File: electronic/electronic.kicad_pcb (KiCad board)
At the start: 2 copper layers, 73.5 x 73 mm, 30 parts, among them IC1 AS5600-ASOT, IC2 AS5600-ASOT, IC3 AS5600-ASOT, IC4 AS5600-ASOT, J2 BAT_AX, M1 ESC, M2 ESC, M3 ESC, M4 ESC, U1 ESP32-DEVKITC-V4, U13 SSD1306, U15 HC-SR04, U16 HC-SR04, U17 HC-SR04, U18 HC-SR04, U2 NEO-6M-GPS, U3 MPU-9250+BMP280, U4 TCA9548AMRGER

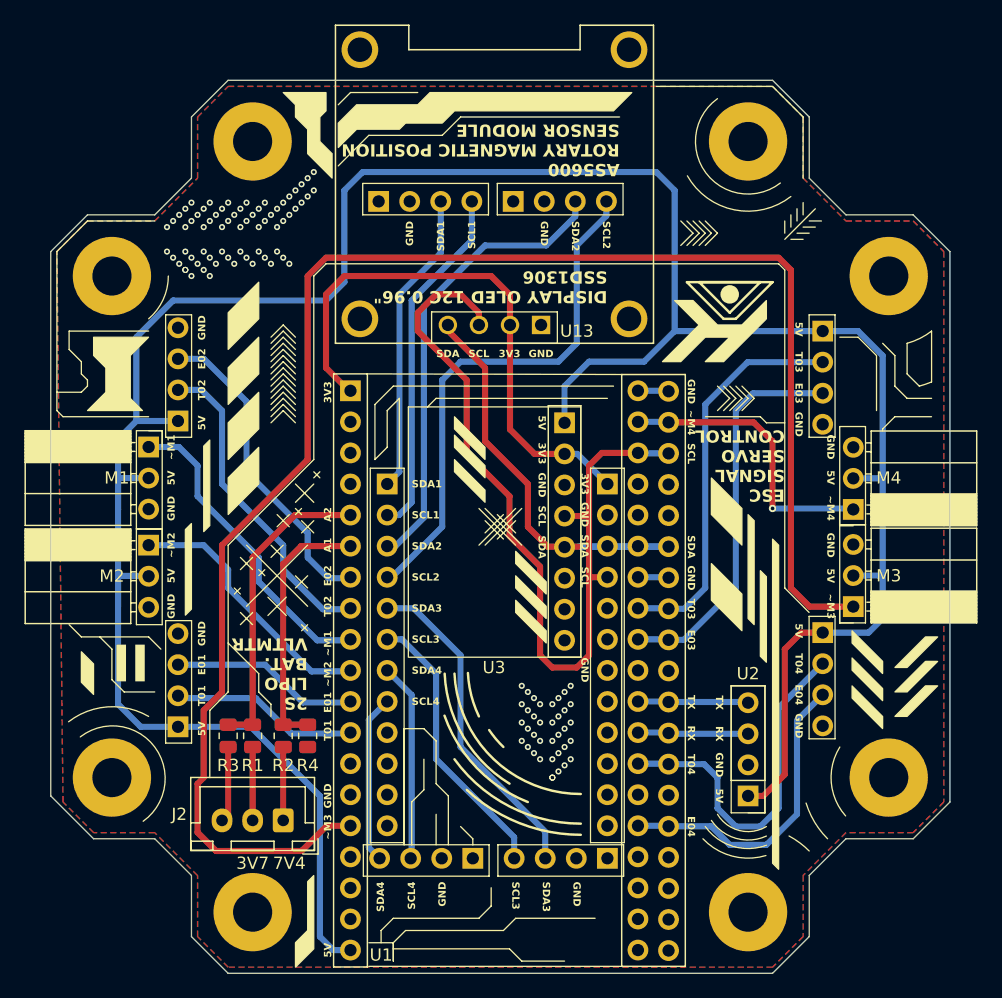
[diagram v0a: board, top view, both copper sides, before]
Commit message: refactor: update PCB
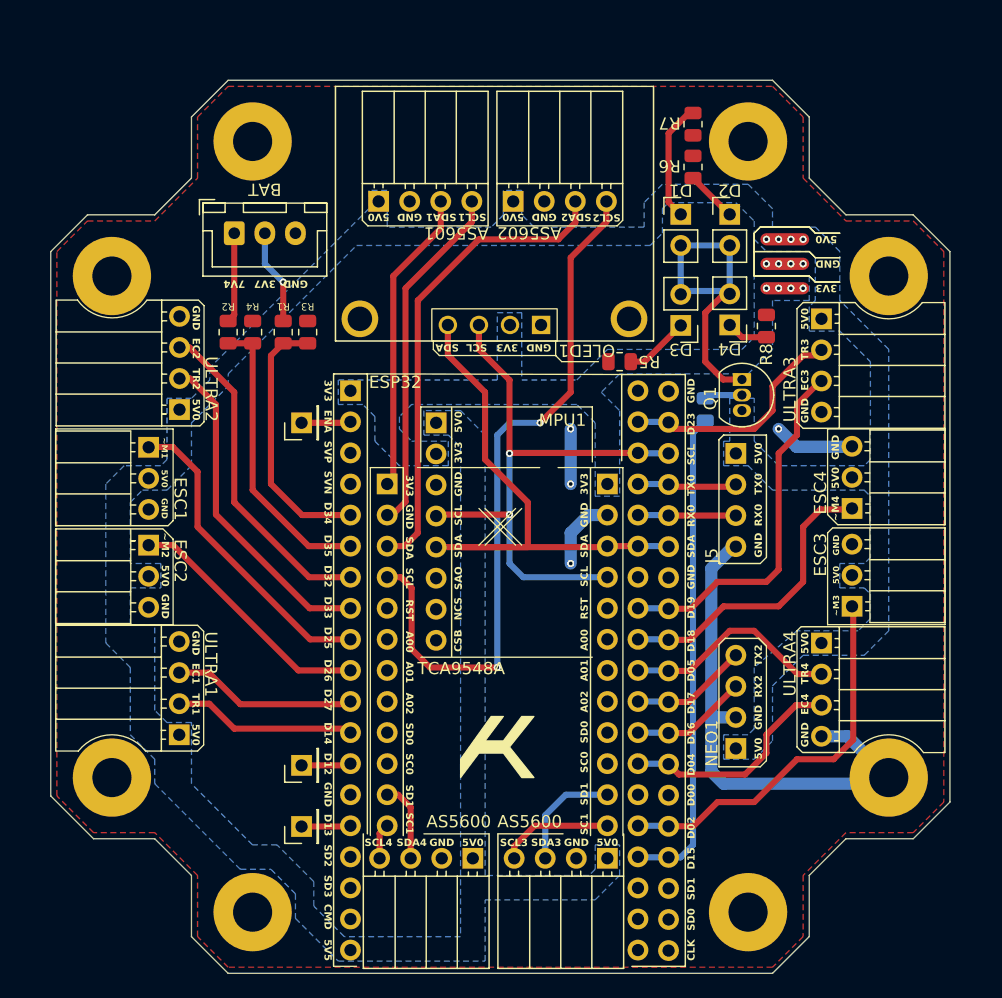
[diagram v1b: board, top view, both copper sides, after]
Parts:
- removed M1, M2, M3, M4: ESC, Connector_PinSocket_2.54mm:PinSocket_1x03_P2.54mm_Horizontal
- added D1: LED, Connector_PinHeader_2.54mm:PinHeader_1x02_P2.54mm_Vertical, F.Cu at (90.0, 61.0)
- added D2: LED, Connector_PinHeader_2.54mm:PinHeader_1x02_P2.54mm_Vertical, F.Cu at (94.0, 61.0)
- added D3: LED, Connector_PinHeader_2.54mm:PinHeader_1x02_P2.54mm_Vertical, F.Cu at (90.0, 70.0)
- added D4: LED, Connector_PinHeader_2.54mm:PinHeader_1x02_P2.54mm_Vertical, F.Cu at (94.0, 70.0)
- added ESC1: ESC, MYPCB:ESC1, F.Cu at (46.5, 80.0)
- added ESC2: ESC, MYPCB:ESC2, F.Cu at (46.5, 88.0)
- added ESC3: ESC, MYPCB:ESC3, F.Cu at (104.0, 93.0)
- added ESC4: ESC, MYPCB:ESC4, F.Cu at (104.0, 85.0)
- added J1: Conn_01x01, Connector_PinHeader_2.54mm:PinHeader_1x01_P2.54mm_Vertical, F.Cu at (59.0, 106.0)
- added J3: Conn_01x01, Connector_PinHeader_2.54mm:PinHeader_1x01_P2.54mm_Vertical, F.Cu at (59.0, 111.0)
- added J4: Conn_01x01, Connector_PinHeader_2.54mm:PinHeader_1x01_P2.54mm_Vertical, F.Cu at (59.0, 78.0)
- added J5: Conn_01x02, Connector_PinHeader_2.54mm:PinHeader_1x04_P2.54mm_Vertical, F.Cu at (94.5, 80.5)
- added Q1: 2222A, Package_TO_SOT_THT:TO-92_Inline, F.Cu at (95.0, 74.5)
- added R5: 220, Resistor_SMD:R_0805_2012Metric, F.Cu at (85.0, 73.0)
- added R6: 220, Resistor_SMD:R_0805_2012Metric, F.Cu at (91.0, 57.1)
- added R7: 220, Resistor_SMD:R_0805_2012Metric, F.Cu at (91.0, 53.6)
- added R8: 220, Resistor_SMD:R_0805_2012Metric, F.Cu at (97.0, 70.1)
- added R9: 330, Resistor_SMD:R_0805_2012Metric, B.Cu at (92.0, 76.9)
- BAT1: renamed from J2; value BAT_AX -> BAT
- MPU1: renamed from U3; value MPU-9250+BMP280 -> MPU+BMP280
- NEO1: renamed from U2; value NEO-6M-GPS -> NEO6M-GPS
- OLED1: renamed from U13; value SSD1306 -> OLED DISPLAY
- moved BAT1 48.2 mm to (53.5, 62.5), turned to 0 degrees
- moved R3 33.6 mm to (59.5, 70.6), turned to 90 degrees
- moved R2 33.3 mm to (53.0, 70.6)
- moved R4 33.3 mm to (55.0, 70.6), turned to 90 degrees
- moved R1 33.1 mm to (57.5, 70.6)
- moved NEO1 4.01 mm to (94.5, 104.6)
- moved MPU1 1.04 mm to (75.8, 86.7)
- moved ULTRA3 1.00 mm to (101.5, 69.5)
- moved ULTRA2 0.94 mm to (49.0, 76.9)
- moved ULTRA4 0.86 mm to (101.5, 96.0)
- moved ULTRA1 0.66 mm to (49.0, 103.5)
- renumbered IC1 to AS1, IC2 to AS2, IC3 to AS3, IC4 to AS4, U4 to TCA1, U15 to ULTRA1, U16 to ULTRA2, U17 to ULTRA3, U18 to ULTRA4
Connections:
- AS1 pad 1: unconnected-(IC1-VDD3V3-Pad1) -> +5V
- AS2 pad 1: unconnected-(IC2-VDD3V3-Pad1) -> +5V
- AS3 pad 1: unconnected-(IC3-VDD3V3-Pad1) -> +5V
- AS4 pad 1: unconnected-(IC4-VDD3V3-Pad1) -> +5V
- BAT1 pad 1: Net-(J2-Pin_1) -> Net-(BAT1-Pin_1)
- BAT1 pad 2: Net-(J2-Pin_2) -> Net-(BAT1-Pin_2)
- R1 pad 1: Net-(J2-Pin_2) -> A02
- R1 pad 2: A02 -> Net-(BAT1-Pin_2)
- R2 pad 1: Net-(J2-Pin_1) -> A01
- R2 pad 2: A01 -> Net-(BAT1-Pin_1)
- REF** pad 1: (no net) -> Earth (x8)
- TCA1 pad 11: unconnected-(U4-SD1-Pad11) -> SW_DA03
- TCA1 pad 12: unconnected-(U4-SC1-Pad12) -> SW_CL03
- TCA1 pad 17: SW_DA03 -> unconnected-(TCA1-SD4-Pad17)
- TCA1 pad 18: SW_CL03 -> unconnected-(TCA1-SC4-Pad18)
- TCA1 pad 19: SW_DA04 -> unconnected-(TCA1-SD5-Pad19)
- TCA1 pad 20: SW_CL04 -> unconnected-(TCA1-SC5-Pad20)
- TCA1 pad 23: unconnected-(U4-SD7-Pad23) -> SW_DA04
- TCA1 pad 24: unconnected-(U4-SC7-Pad24) -> SW_CL04
- U1 pad 13: unconnected-(U1-IO12-Pad13) -> Net-(J1-Pin_1)
- U1 pad 15: M3_SIGN -> Net-(J3-Pin_1)
- U1 pad 2: unconnected-(U1-EN-Pad2) -> Net-(J4-Pin_1)
- U1 pad 21: M4_SIGN -> CH_T03
- U1 pad 23: unconnected-(U1-TXD0-Pad23) -> Net-(J5-Pin_2)
- U1 pad 24: unconnected-(U1-RXD0-Pad24) -> Net-(J5-Pin_3)
- U1 pad 27: CH_T03 -> CH_E03
- U1 pad 28: CH_E03 -> M4_SIGN
- U1 pad 29: unconnected-(U1-IO5-Pad29) -> CH_T04
- U1 pad 32: CH_T04 -> CH_E04
- U1 pad 34: CH_E04 -> M3_SIGN
- U1 pad 35: unconnected-(U1-IO15-Pad35)_1 -> LEDS
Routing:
- net +5V: track 225.7 -> 3.08 mm, vias 0 -> 4
- net M3_SIGN: track 135.5 -> 31.4 mm
- net Earth: track 10.7 -> 63.4 mm, vias 0 -> 8
- net +3.3V: track 45.9 -> 3.12 mm, vias 0 -> 4
- net LEDS: track 0.00 -> 40.1 mm
- net Net-(D1-A): track 0.00 -> 25.7 mm
- net IMU_SCL: track 71.8 -> 48.1 mm, vias 0 -> 2
- net SW_DA03: track 27.1 -> 9.30 mm
- net SW_CL02: track 43.1 -> 58.2 mm, vias 0 -> 2
- net CH_T03: track 32.3 -> 18.5 mm
- net SW_CL03: track 22.9 -> 9.30 mm
- net CH_T04: track 29.0 -> 17.1 mm
- net SW_CL04: track 13.8 -> 2.94 mm
- net Net-(D1-K): track 0.00 -> 9.73 mm
- net SW_DA04: track 16.2 -> 6.52 mm
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- added copper zone on B.Cu, net +3.3V
- added copper zone on B.Cu, net +5V
- removed copper zone on B.Cu, net Earth
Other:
- board text added: "5V0"
- board text removed: "2S LIPO BAT. VLTMTR"
- board text removed: "3V7"
- board text removed: "7V4"
- board text removed: "A1"
- board text removed: "A2"
- board text removed: "AK VANT II"
- board text removed: "AS5600 ROTARY MAGNETIC POSITION SENSOR MODULE"
- board text removed: "DISPLAY OLED 12C 0.96{dblquote} SSD1306"
- board text removed: "E01"
- board text removed: "E02"
- board text removed: "E03"
- board text removed: "E04"
- board text removed: "ESC SIGNAL SERVO CONTROL"
- board text removed: "II"
- board text removed: "J2"
- board text removed: "RX"
- board text removed: "SCL"
- board text removed: "SCL1"
- board text removed: "SCL2"
- board text removed: "SCL3"
- board text removed: "SCL4"
- board text removed: "SDA"
- board text removed: "SDA1"
- board text removed: "SDA2"
- board text removed: "SDA3"
- board text removed: "SDA4"
- board text removed: "T01"
- board text removed: "T02"
- board text removed: "T03"
- board text removed: "T04"
- board text removed: "TX"
- board text removed: "~M1"
- board text removed: "~M3"
- board text removed: "~M4"
